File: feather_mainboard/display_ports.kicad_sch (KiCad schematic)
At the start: 1 part, among them J1 61300811121

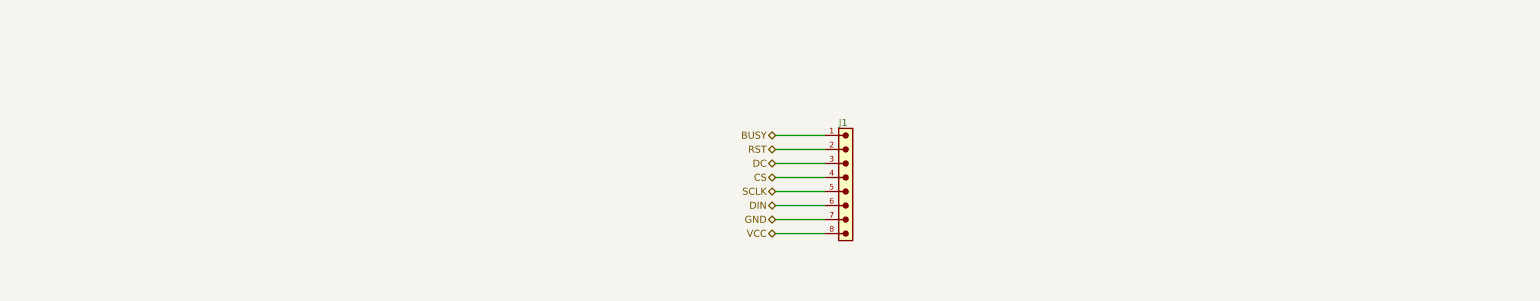
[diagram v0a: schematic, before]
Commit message: finished daughter board
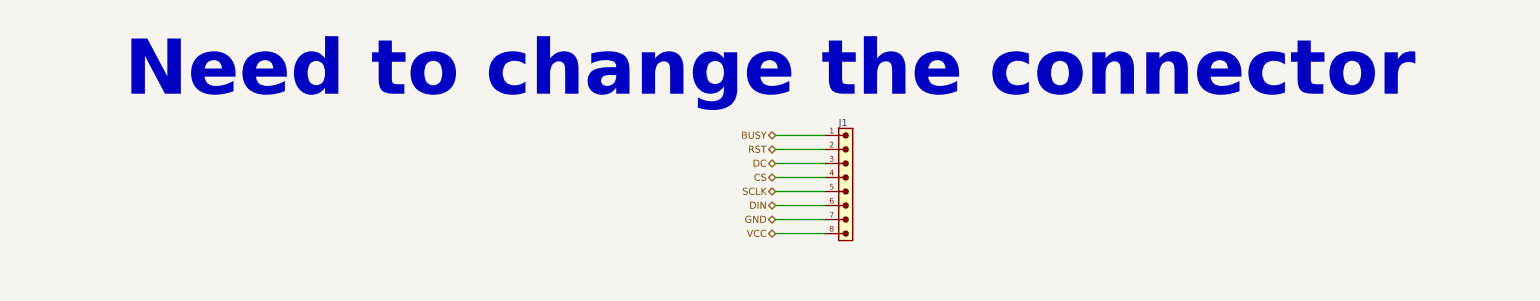
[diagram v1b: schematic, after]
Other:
- note added: "Need to change the connector"
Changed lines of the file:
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@@
+		)
+	)
+	(text "Need to change the connector"
+		(exclude_from_sim no)
+		(at 138.684 70.612 0)
+		(effects
+			(font
+				(size 10 10)
+				(thickness 4)
+				(bold yes)
+			)
 		)
 	)

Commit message: finished mainboard design, need to do the routing
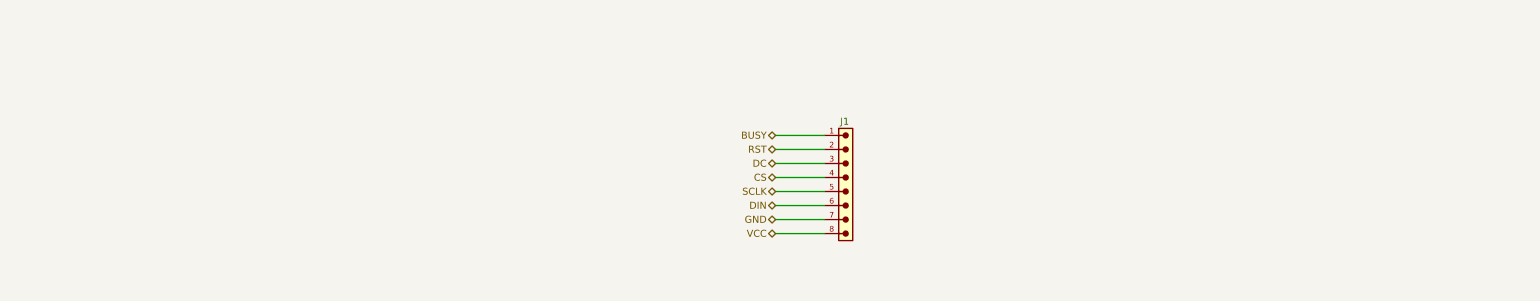
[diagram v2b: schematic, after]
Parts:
- removed J1: 61300811121, Custom footprints:61300811121, symbol 6130XX11121_61300811121:6130XX11121_61300811121
- added J1: 61900819521, Custom footprints:61900819521, symbol 61900819521:61900819521
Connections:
- net BUSY: now also J1.1
- net CS: now also J1.4
- net DC: now also J1.3
- net DIN: now also J1.6
- net GND: now also J1.7
- net RST: now also J1.2
- net SCLK: now also J1.5
- net VCC: now also J1.8
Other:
- note removed: "Need to change the connector"
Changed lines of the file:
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@@
-		)
-	)
-	(text "Need to change the connector"
-		(exclude_from_sim no)
-		(at 138.684 70.612 0)
-		(effects
-			(font
-				(size 10 10)
-				(thickness 4)
-				(bold yes)
-			)
 		)
 	)
@@
 	)
 	(symbol
-		(lib_id "6130XX11121_61300811121:6130XX11121_61300811121")
+		(lib_id "61900819521:61900819521")
 		(at 153.67 90.17 270)
 		(unit 1)
@@
 		(dnp no)
 		(property "Reference" "J1"
-			(at 151.13 80.264 90)
+			(at 151.384 80.01 90)
 			(effects
 				(font
@@
 			)
 		)
-		(property "Value" "61300811121"
-			(at 146.812 79.248 90)
-			(effects
-				(font
-					(size 1.27 1.27)
-				)
-				(justify left)
-				(hide yes)
-			)
-		)
-		(property "Footprint" "Custom footprints:61300811121"
+		(property "Value" "61900819521"
+			(at 153.67 90.17 0)
+			(effects
+				(font
+					(size 1.27 1.27)
+				)
+				(justify bottom)
+				(hide yes)
+			)
+		)
+		(property "Footprint" "Custom footprints:61900819521"
 			(at 153.67 90.17 0)
 			(effects
@@
 			)
 		)
-		(property "ROWS" "Single"
-			(at 153.67 90.17 0)
-			(effects
-				(font
-					(size 1.27 1.27)
-				)
-				(justify bottom)
-				(hide yes)
-			)
-		)
-		(property "GENDER" "Pin Header"
+		(property "MF" "Würth Elektronik"
+			(at 153.67 90.17 0)
+			(effects
+				(font
+					(size 1.27 1.27)
+				)
+				(justify bottom)
+				(hide yes)
+			)
+		)
+		(property "CONTACT-RESISTANCE" "20mOhm"
+			(at 153.67 90.17 0)
+			(effects
+				(font
+					(size 1.27 1.27)
+				)
+				(justify bottom)
+				(hide yes)
+			)
+		)
+		(property "Description_1" "\n                        \n                            EMI Gaskets, Sheets, Absorbers & Shielding\n                        \n"
+			(at 153.67 90.17 0)
+			(effects
+				(font
+					(size 1.27 1.27)
+				)
+				(justify bottom)
+				(hide yes)
+			)
+		)
+		(property "Package" "None"
+			(at 153.67 90.17 0)
+			(effects
+				(font
+					(size 1.27 1.27)
+				)
+				(justify bottom)
+				(hide yes)
+			)
+		)
+		(property "GENDER" "Male"
 			(at 153.67 90.17 0)
 			(effects
@@
 			)
 		)
-		(property "IR" "3A"
-			(at 153.67 90.17 0)
-			(effects
-				(font
-					(size 1.27 1.27)
-				)
-				(justify bottom)
-				(hide yes)
-			)
-		)
-		(property "VALUE" "61300811121"
+		(property "PITCH" "2.54mm"
+			(at 153.67 90.17 0)
+			(effects
+				(font
+					(size 1.27 1.27)
+				)
+				(justify bottom)
+				(hide yes)
+			)
+		)
+		(property "Check_prices" "https://www.snapeda.com/parts/61900819521/Wurth+Elektronik/view-part/?ref=eda"
+			(at 153.67 90.17 0)
+			(effects
+				(font
+					(size 1.27 1.27)
+				)
+				(justify bottom)
+				(hide yes)
+			)
+		)
+		(property "L" "20.32mm"
+			(at 153.67 90.17 0)
+			(effects
+				(font
+					(size 1.27 1.27)
+				)
+				(justify bottom)
+				(hide yes)
+			)
+		)
+		(property "Price" "None"
 			(at 153.67 90.17 0)
 			(effects
@@
 			)
 		)
+		(property "PART-NUMBER" "61900819521"
+			(at 153.67 90.17 0)
+			(effects
+				(font
+					(size 1.27 1.27)
+				)
+				(justify bottom)
+				(hide yes)
+			)
+		)
+		(property "SnapEDA_Link" "https://www.snapeda.com/parts/61900819521/Wurth+Elektronik/view-part/?ref=snap"
+			(at 153.67 90.17 0)
+			(effects
+				(font
+					(size 1.27 1.27)
+				)
+				(justify bottom)
+				(hide yes)
+			)
+		)
+		(property "DATASHEET-URL" "https://www.we-online.com/redexpert/spec/61900819521?ae"
+			(at 153.67 90.17 0)
+			(effects
+				(font
+					(size 1.27 1.27)
+				)
+				(justify bottom)
+				(hide yes)
+			)
+		)
+		(property "MP" "61900819521"
+			(at 153.67 90.17 0)
+			(effects
+				(font
+					(size 1.27 1.27)
+				)
+				(justify bottom)
+				(hide yes)
+			)
+		)
+		(property "WORKING-VOLTAGE" "250V(AC)"
+			(at 153.67 90.17 0)
+			(effects
+				(font
+					(size 1.27 1.27)
+				)
+				(justify bottom)
+				(hide yes)
+			)
+		)
 		(property "PINS" "8"
 			(at 153.67 90.17 0)
@@
 			)
 		)
-		(property "DATASHEET-URL" "https://www.we-online.com/redexpert/spec/61300811121?ae"
-			(at 153.67 90.17 0)
-			(effects
-				(font
-					(size 1.27 1.27)
-				)
-				(justify bottom)
-				(hide yes)
-			)
-		)
-		(property "PITCH" "2.54mm"
-			(at 153.67 90.17 0)
-			(effects
-				(font
-					(size 1.27 1.27)
-				)
-				(justify bottom)
-				(hide yes)
-			)
-		)
-		(property "PART-NUMBER" "61300811121"
-			(at 153.67 90.17 0)
-			(effects
-				(font
-					(size 1.27 1.27)
-				)
-				(justify bottom)
-				(hide yes)
-			)
-		)
-		(property "TYPE" "Straight"
-			(at 153.67 90.17 0)
-			(effects
-				(font
-					(size 1.27 1.27)
-				)
-				(justify bottom)
-				(hide yes)
-			)
+		(property "TYPE" "Right Angled Top Locking"
+			(at 153.67 90.17 0)
+			(effects
+				(font
+					(size 1.27 1.27)
+				)
+				(justify bottom)
+				(hide yes)
+			)
+		)
+		(property "PCB-CABLE-PANEL" "PCB"
+			(at 153.67 90.17 0)
+			(effects
+				(font
+					(size 1.27 1.27)
+				)
+				(justify bottom)
+				(hide yes)
+			)
+		)
+		(property "Availability" "In Stock"
+			(at 153.67 90.17 0)
+			(effects
+				(font
+					(size 1.27 1.27)
+				)
+				(justify bottom)
+				(hide yes)
+			)
+		)
+		(pin "6"
+		)
+		(pin "5"
 		)
 		(pin "2"
 		)
-		(pin "5"
+		(pin "1"
+		)
+		(pin "8"
+		)
+		(pin "3"
 		)
 		(pin "7"
 		)
-		(pin "3"
-		)
-		(pin "6"
-		)
-		(pin "1"
-		)
-		(pin "8"
-		)
 		(pin "4"

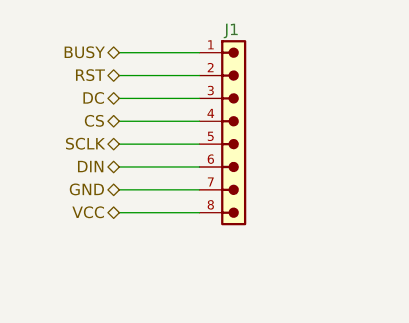
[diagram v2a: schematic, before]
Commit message: finished mainboard and daughterboard
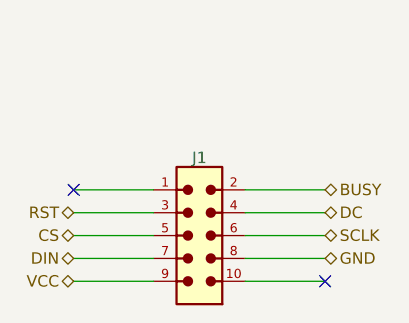
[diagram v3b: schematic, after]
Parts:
- removed J1: 61900819521, Custom footprints:61900819521, symbol 61900819521:61900819521
- added J1: 62501021721, Custom footprints:62501021721, symbol 6250XX21721_62501021721:6250XX21721_62501021721
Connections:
- net BUSY: now also J1.2
- net CS: now also J1.5
- net DC: now also J1.4
- net DIN: now also J1.7
- net GND: now also J1.8
- net RST: now also J1.3
- net SCLK: now also J1.6
- net VCC: now also J1.9
- no-connect marks 0 -> 2
